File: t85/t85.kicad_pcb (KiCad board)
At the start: 2 copper layers, 20.3 x 7.6 mm, 15 parts, among them J1 USB, J2 Conn_02x04_Counter_Clockwise, SW1 SW_Push, U1 ATtiny85-20S

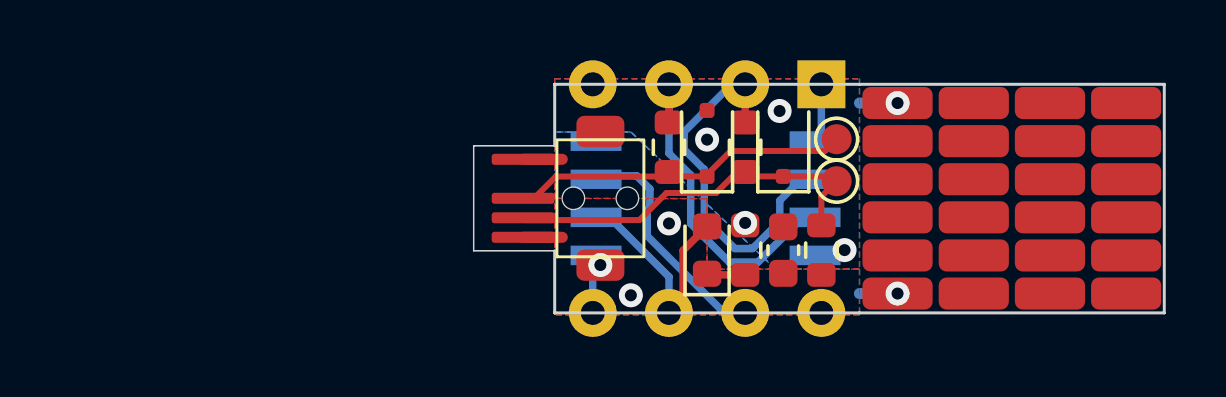
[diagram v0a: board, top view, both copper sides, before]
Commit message: -
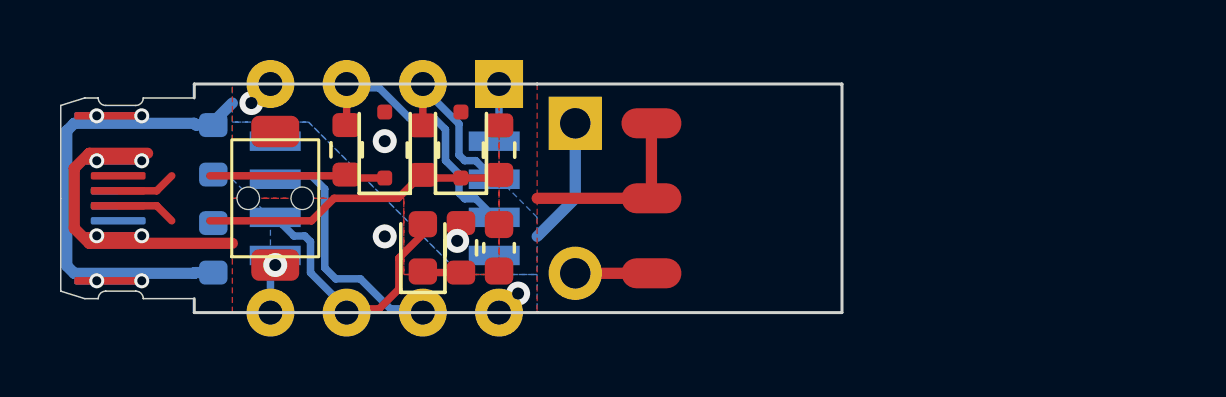
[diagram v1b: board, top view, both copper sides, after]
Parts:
- removed REF**: smd_3x4, Library:smd_3x4
- removed TP1, TP2: TestPoint, TestPoint:TestPoint_Pad_D1.0mm
- added C2: 1F5, Library:edlc, F.Cu at (112.7, 100.0)
- added R5: 5k1, Resistor_SMD:R_0603_1608Metric, B.Cu at (100.6, 98.4)
- added R6: 5k1, Resistor_SMD:R_0603_1608Metric, B.Cu at (100.6, 101.7)
- added SW2: SW_SPDT, Library:sw, F.Cu at (115.2, 100.0)
- J1: value USB -> USB-C; footprint Library:USB-micro-b -> Library:USB-C
- J2: value Conn_02x04_Counter_Clockwise -> OUT
- moved J1 12.0 mm to (100.0, 100.0)
- moved R4 11.2 mm to (110.2, 98.4)
- moved SW1 10.8 mm to (102.7, 100.0)
- moved R2 10.7 mm to (107.6, 98.4), turned to -90 degrees
- moved R3 10.7 mm to (105.1, 98.4)
- moved D2 10.7 mm to (106.3, 98.2)
- moved D3 10.7 mm to (108.9, 98.2)
- moved J2 10.7 mm to (110.2, 96.2)
- moved U1 10.7 mm to (106.3, 100.0)
- moved C1 9.47 mm to (110.2, 101.7)
- moved R1 9.47 mm to (108.9, 101.7)
- moved D1 9.47 mm to (107.6, 101.7)
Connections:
- net RESET# renamed EN
- C1 pad 1: +5V -> VCC
- J1 pad 4: +5V -> VCC
- J2 pad 8: +5V -> VCC
- R2 pad 1: D- -> PB3
- R2 pad 2: PB3 -> D-
- R4 pad 1: D- -> VCC
- R4 pad 2: +5V -> D-
- U1 pad 8: +5V -> VCC
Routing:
- net GND: track 2.57 -> 19.8 mm, vias 5 -> 7
- net VCC: track 0.00 -> 16.4 mm, vias 0 -> 6
- net PB3: track 12.4 -> 5.40 mm
- net D+: track 11.4 -> 7.92 mm
- net +5V: track 2.57 -> 0.00 mm, vias 3 -> 0
- net /Vedlc: track 0.00 -> 2.54 mm
- net PB4: track 11.3 -> 8.83 mm
- net PB1: track 7.69 -> 8.76 mm
- net D-: track 13.0 -> 12.4 mm
- added copper zone on B.Cu, net VCC
- added copper zone on F.Cu, net VCC
- removed copper zone on B.Cu, net +5V
- removed copper zone on F.Cu, net +5V
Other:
- board size 20.3 x 7.6 mm -> 21.6 x 7.6 mm
